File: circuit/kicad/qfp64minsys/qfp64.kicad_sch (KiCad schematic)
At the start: 0 parts

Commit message: Progress
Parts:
- added C1, C2, C4: 100nF, Capacitor_SMD:C_0805_2012Metric_Pad1.18x1.45mm_HandSolder, symbol Device:C
- added C3: 100uF, Capacitor_THT:CP_Radial_D4.0mm_P1.50mm, symbol Device:C_Polarized
- added C5, C6, C7, C8: 10nF, Capacitor_SMD:C_0805_2012Metric_Pad1.18x1.45mm_HandSolder, symbol Device:C
- added C9: 4u7F, Capacitor_Tantalum_SMD:CP_EIA-3216-18_Kemet-A, symbol Device:C
- added D1: RED, LED_SMD:LED_0805_2012Metric_Pad1.15x1.40mm_HandSolder, symbol Device:LED
- added D2: YELLOW, LED_SMD:LED_0805_2012Metric_Pad1.15x1.40mm_HandSolder, symbol Device:LED
- added J1, J6: Conn_01x05_Pin, Connector_PinSocket_2.54mm:PinSocket_1x05_P2.54mm_Vertical, symbol Connector:Conn_01x05_Pin
- added J10, J7, J9: Conn_01x09_Pin, Connector_PinSocket_2.54mm:PinSocket_1x09_P2.54mm_Vertical, symbol Connector:Conn_01x09_Pin
- added J2, J3: USB_B_Mini, Connector_USB:USB_Mini-B_Wuerth_65100516121_Horizontal, symbol Connector:USB_B_Mini
- added J4, J5: Conn_01x03_Pin, Connector_PinSocket_2.54mm:PinSocket_1x03_P2.54mm_Vertical, symbol Connector:Conn_01x03_Pin
- added J8: Conn_01x12_Pin, Connector_PinSocket_2.54mm:PinSocket_1x12_P2.54mm_Vertical, symbol Connector:Conn_01x12_Pin
- added JP1, JP2, JP3, JP4, JP5: SolderJumper_2_Open, Jumper:SolderJumper-2_P1.3mm_Open_TrianglePad1.0x1.5mm, symbol Jumper:SolderJumper_2_Open
- added R1, R2, R3, R6: 10K, Resistor_SMD:R_0805_2012Metric_Pad1.20x1.40mm_HandSolder, symbol Device:R
- added R4, R5: 330, Resistor_SMD:R_0805_2012Metric_Pad1.20x1.40mm_HandSolder, symbol Device:R
- added SW1, SW2, SW3: SW_Push, Button_Switch_THT:SW_PUSH_6mm, symbol Switch:SW_Push
- added U1: STM32F401RETx, Package_QFP:LQFP-64_10x10mm_P0.5mm, symbol MCU_ST_STM32F4:STM32F401RETx
- added U2: CH340C, Package_SO:SOIC-16_3.9x9.9mm_P1.27mm, symbol Interface_USB:CH340C
- added U3: AMS1117-3.3, Package_TO_SOT_SMD:SOT-223-3_TabPin2, symbol Regulator_Linear:AMS1117-3.3
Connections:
- new net: D2.2 (A), R5.2
- new net: JP1.1 (A), U1.19 (VDD)
- new net: C1.1, U2.4 (V3)
- new net: J3.3 (D+), U2.5 (UD+)
- new net: J3.2 (D-), U2.6 (UD-)
- new net: JP2.1 (A), U1.48 (VDD)
- new net: J6.1 (Pin_1), JP3.1 (A)
- new net: J6.2 (Pin_2), JP4.1 (A)
- new net: D1.2 (A), R4.2
- new net +5V: C3.1, J2.1 (VBUS), J3.1 (VBUS), J4.1 (Pin_1), J4.2 (Pin_2), J4.3 (Pin_3), JP3.2 (B), U2.16 (VCC), U3.3 (VI)
- new net BOOT0: R2.2, SW2.2, U1.60 (BOOT0)
- new net BOOT1: JP5.1 (A), U1.28 (PB2)
- new net BTN: R3.2, SW3.2, U1.2 (PC13)
- new net GND: C1.2, C2.2, C3.2, C4.2, C5.2, C6.2, C7.2, C8.2, C9.2, D1.1 (K), J1.3 (Pin_3), J2.5 (GND), J2.6 (Shield), J3.5 (GND), J3.6 (Shield), J5.1 (Pin_1), J5.2 (Pin_2), J5.3 (Pin_3), J6.5 (Pin_5), JP5.2 (B), SW1.1, SW2.1, SW3.1, U1.12 (VSSA), U1.18 (VSS), U1.31 (VSS), U1.47 (VSS), U1.63 (VSS), U2.1 (GND), U3.1 (GND)
- new net LED: D2.1 (K), U1.21 (PA5)
- new net NRST: J1.5 (Pin_5), R1.2, SW1.2, U1.7 (NRST)
- new net PA0: J9.7 (Pin_7), U1.14 (PA0)
- new net PA1: J9.8 (Pin_8), U1.15 (PA1)
- new net PA15: J8.1 (Pin_1), U1.50 (PA15)
- new net PA2: J9.9 (Pin_9), U1.16 (PA2)
- new net PA3: J10.1 (Pin_1), U1.17 (PA3)
- new net PA4: J10.2 (Pin_2), U1.20 (PA4)
- new net PA6: J10.3 (Pin_3), U1.22 (PA6)
- new net PA7: J10.4 (Pin_4), U1.23 (PA7)
- new net PA8: J7.1 (Pin_1), U1.41 (PA8)
- new net PB0: J10.7 (Pin_7), U1.26 (PB0)
- new net PB1: J10.8 (Pin_8), U1.27 (PB1)
- new net PB10: J10.9 (Pin_9), U1.29 (PB10)
- new net PB12: J7.9 (Pin_9), U1.33 (PB12)
- new net PB13: J7.8 (Pin_8), U1.34 (PB13)
- new net PB14: J7.7 (Pin_7), U1.35 (PB14)
- new net PB15: J7.6 (Pin_6), U1.36 (PB15)
- new net PB3: J8.6 (Pin_6), U1.55 (PB3)
- new net PB4: J8.7 (Pin_7), U1.56 (PB4)
- new net PB5: J8.8 (Pin_8), U1.57 (PB5)
- new net PB6: J8.9 (Pin_9), U1.58 (PB6)
- new net PB7: J8.10 (Pin_10), U1.59 (PB7)
- new net PB8: J8.11 (Pin_11), U1.61 (PB8)
- new net PB9: J8.12 (Pin_12), U1.62 (PB9)
- new net PC0: J9.3 (Pin_3), U1.8 (PC0)
- new net PC1: J9.4 (Pin_4), U1.9 (PC1)
- new net PC10: J8.2 (Pin_2), U1.51 (PC10)
- new net PC11: J8.3 (Pin_3), U1.52 (PC11)
- new net PC12: J8.4 (Pin_4), U1.53 (PC12)
- new net PC14: J9.1 (Pin_1), U1.3 (PC14)
- new net PC15: J9.2 (Pin_2), U1.4 (PC15)
- new net PC2: J9.5 (Pin_5), U1.10 (PC2)
- new net PC3: J9.6 (Pin_6), U1.11 (PC3)
- new net PC4: J10.5 (Pin_5), U1.24 (PC4)
- new net PC5: J10.6 (Pin_6), U1.25 (PC5)
- new net PC6: J7.5 (Pin_5), U1.37 (PC6)
- new net PC7: J7.4 (Pin_4), U1.38 (PC7)
- new net PC8: J7.3 (Pin_3), U1.39 (PC8)
- new net PC9: J7.2 (Pin_2), U1.40 (PC9)
- new net PD2: J8.5 (Pin_5), U1.54 (PD2)
- new net RXD: J6.4 (Pin_4), U1.43 (PA10), U2.2 (TXD)
- new net SWCLK: J1.2 (Pin_2), U1.49 (PA14)
- new net SWDIO: J1.4 (Pin_4), U1.46 (PA13)
- new net TXD: J6.3 (Pin_3), U1.42 (PA9), U2.3 (RXD)
- new net USBDM: J2.2 (D-), U1.44 (PA11)
- new net USBDP: J2.3 (D+), R6.2, U1.45 (PA12)
- new net VCAP: C9.1, U1.30 (VCAP1)
- new net VDD: C2.1, C4.1, C5.1, C6.1, C7.1, C8.1, J1.1 (Pin_1), JP1.2 (B), JP2.2 (B), JP4.2 (B), R1.1, R2.1, R3.1, R4.1, R5.1, R6.1, U1.1 (VBAT), U1.13 (VREF+), U1.32 (VDD), U1.64 (VDD), U3.2 (VO)
- no-connect marks 0 -> 11

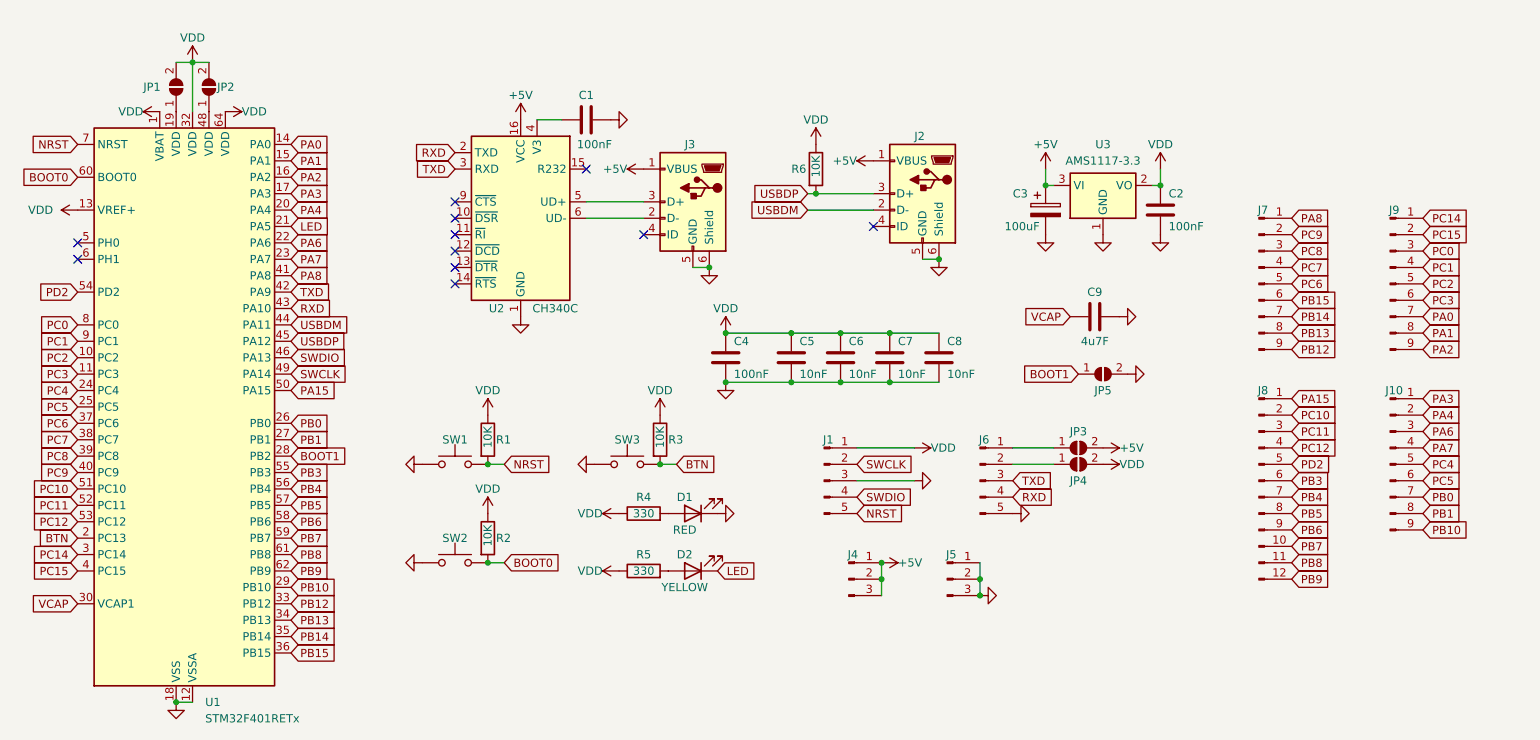
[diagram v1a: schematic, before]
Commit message: Coba Pesan
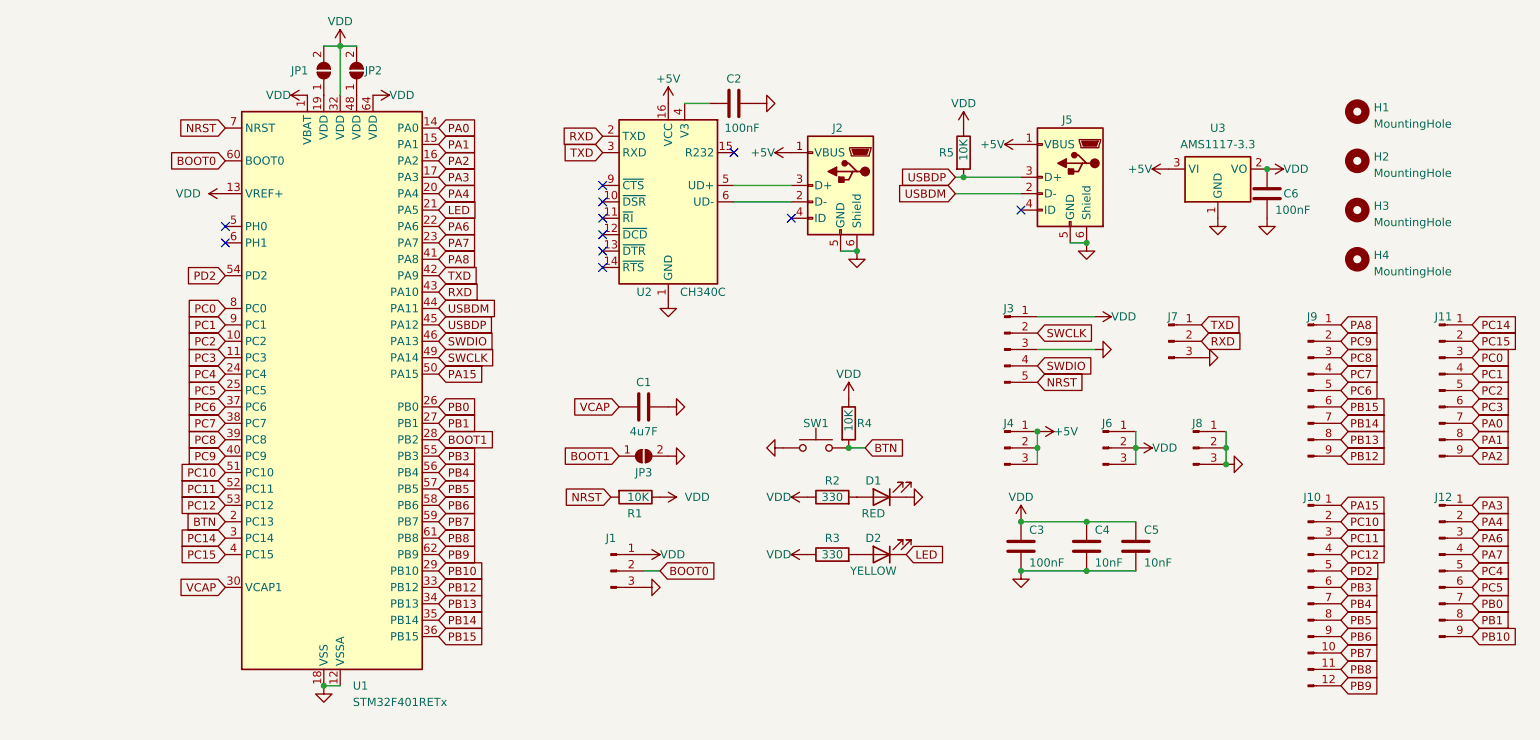
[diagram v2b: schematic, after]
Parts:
- removed C3: 100uF, Capacitor_THT:CP_Radial_D4.0mm_P1.50mm, symbol Device:C_Polarized
- removed C7, C8: 10nF, Capacitor_SMD:C_0805_2012Metric_Pad1.18x1.45mm_HandSolder, symbol Device:C
- removed J6: Conn_01x05_Pin, Connector_PinSocket_2.54mm:PinSocket_1x05_P2.54mm_Vertical, symbol Connector:Conn_01x05_Pin
- removed JP3, JP4: SolderJumper_2_Open, Jumper:SolderJumper-2_P1.3mm_Open_TrianglePad1.0x1.5mm, symbol Jumper:SolderJumper_2_Open
- removed R2: 10K, Resistor_SMD:R_0805_2012Metric_Pad1.20x1.40mm_HandSolder, symbol Device:R
- removed SW1, SW2: SW_Push, Button_Switch_THT:SW_PUSH_6mm, symbol Switch:SW_Push
- added H1, H2, H3, H4: MountingHole, MountingHole:MountingHole_2.2mm_M2, symbol Mechanical:MountingHole
- added J1, J6, J7: Conn_01x03_Pin, Connector_PinHeader_2.54mm:PinHeader_1x03_P2.54mm_Vertical, symbol Connector:Conn_01x03_Pin
- J10: renamed from J8; footprint Connector_PinSocket_2.54mm:PinSocket_1x12_P2.54mm_Vertical -> Connector_PinHeader_2.54mm:PinHeader_1x12_P2.54mm_Vertical
- J11: renamed from J9; footprint Connector_PinSocket_2.54mm:PinSocket_1x09_P2.54mm_Vertical -> Connector_PinHeader_2.54mm:PinHeader_1x09_P2.54mm_Vertical
- J12: renamed from J10; footprint Connector_PinSocket_2.54mm:PinSocket_1x09_P2.54mm_Vertical -> Connector_PinHeader_2.54mm:PinHeader_1x09_P2.54mm_Vertical
- J3: renamed from J1; footprint Connector_PinSocket_2.54mm:PinSocket_1x05_P2.54mm_Vertical -> Connector_PinHeader_2.54mm:PinHeader_1x05_P2.54mm_Vertical
- J4: footprint Connector_PinSocket_2.54mm:PinSocket_1x03_P2.54mm_Vertical -> Connector_PinHeader_2.54mm:PinHeader_1x03_P2.54mm_Vertical
- J8: renamed from J5; footprint Connector_PinSocket_2.54mm:PinSocket_1x03_P2.54mm_Vertical -> Connector_PinHeader_2.54mm:PinHeader_1x03_P2.54mm_Vertical
- J9: renamed from J7; footprint Connector_PinSocket_2.54mm:PinSocket_1x09_P2.54mm_Vertical -> Connector_PinHeader_2.54mm:PinHeader_1x09_P2.54mm_Vertical
- JP1, JP2: footprint Jumper:SolderJumper-2_P1.3mm_Open_TrianglePad1.0x1.5mm -> Jumper:SolderJumper-2_P1.3mm_Open_RoundedPad1.0x1.5mm
- JP3: renamed from JP5; footprint Jumper:SolderJumper-2_P1.3mm_Open_TrianglePad1.0x1.5mm -> Jumper:SolderJumper-2_P1.3mm_Open_RoundedPad1.0x1.5mm
- renumbered C9 to C1, C1 to C2, C4 to C3, C5 to C4, C6 to C5, C2 to C6, J3 to J2, J2 to J5, R4 to R2, R5 to R3, R3 to R4, R6 to R5, SW3 to SW1
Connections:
- net BOOT0: now also J1.2 (Pin_2)
- net GND: now also J1.3 (Pin_3), J7.3 (Pin_3)
- net RXD: now also J7.2 (Pin_2)
- net TXD: now also J7.1 (Pin_1)
- net VDD: now also J1.1 (Pin_1), J6.1 (Pin_1), J6.2 (Pin_2), J6.3 (Pin_3)
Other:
- moved on the sheet: C1, C2, C3, C4, C5, C6, D1, D2, J10, J11, J12, J2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
